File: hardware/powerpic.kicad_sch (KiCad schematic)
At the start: 21 parts

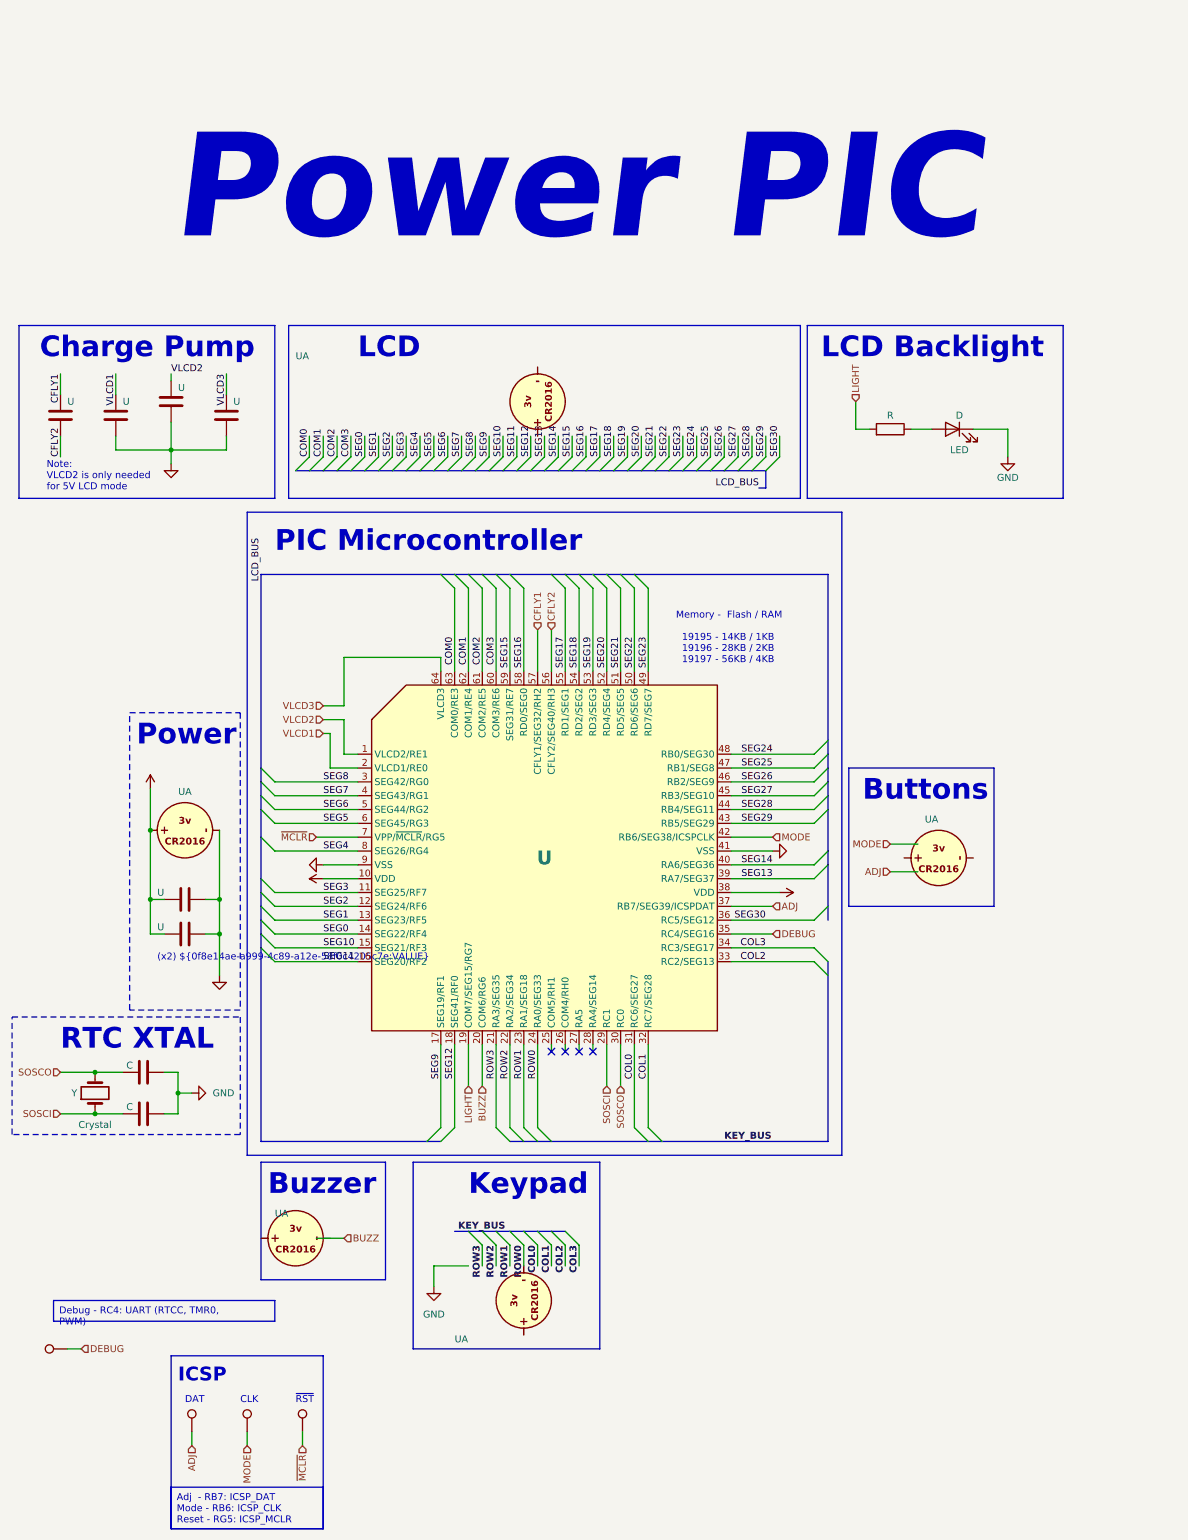
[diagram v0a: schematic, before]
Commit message: release version 2.1
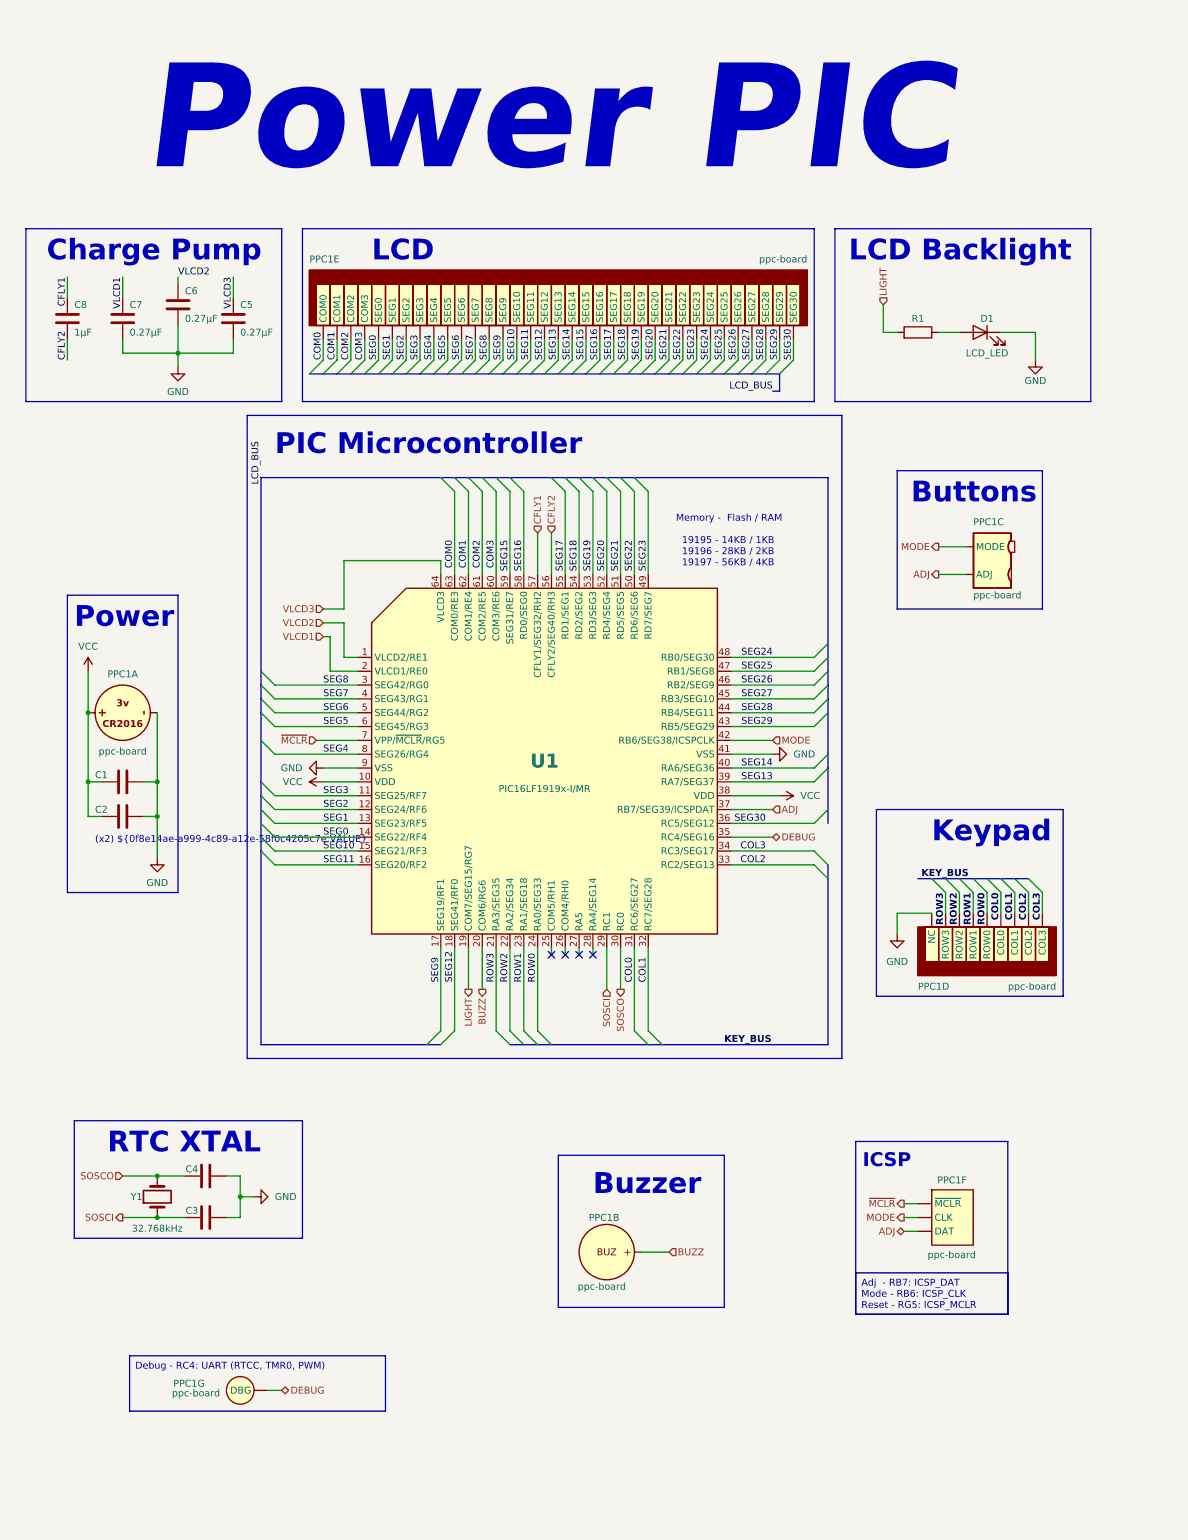
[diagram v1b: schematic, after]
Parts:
- removed TP (x4): TestPoint, symbol Connector:TestPoint
- added unit 7 of PPC1
- added unit 6 of PPC1
- C1, C2: renamed from U; value (none) -> 0.1μF; footprint (none) -> Capacitor_SMD:C_0402_1005Metric
- C3, C4: renamed from C; value C -> TBD; footprint (none) -> Capacitor_SMD:C_0603_1608Metric
- C5, C6, C7: renamed from U; value (none) -> 0.27μF; footprint (none) -> Capacitor_SMD:C_0402_1005Metric
- C8: renamed from U; value (none) -> 1μF; footprint (none) -> Capacitor_SMD:C_0402_1005Metric
- D1: renamed from D; value LED -> LCD_LED; footprint (none) -> LED_SMD:LED_0402_1005Metric
- PPC1: renamed from U; value (none) -> ppc-board; footprint (none) -> ppc-watch:ppc-board
- R1: renamed from R; value R -> TBD; footprint (none) -> Resistor_SMD:R_0603_1608Metric
- U1: renamed from U; value (none) -> PIC16LF1919x-I/MR; footprint (none) -> Package_DFN_QFN:QFN-64-1EP_9x9mm_P0.5mm_EP5.4x5.4mm
- Y1: renamed from Y; value Crystal -> 32.768kHz; footprint (none) -> Crystal:Crystal_SMD_MicroCrystal_CC7V-T1A-2Pin_3.2x1.5mm
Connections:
- net ADJ: now also PPC1.5 (ADJ), PPC1.52 (DAT)
- net BUZZ: now also PPC1.3 (buzz_p)
- net COL0: now also PPC1.11 (COL0)
- net COL1: now also PPC1.12 (COL1)
- net COL2: now also PPC1.13 (COL2)
- net COL3: now also PPC1.14 (COL3)
- net COM0: now also PPC1.15 (COM0)
- net COM1: now also PPC1.16 (COM1)
- net COM2: now also PPC1.17 (COM2)
- net COM3: now also PPC1.18 (COM3)
- net DEBUG: now also PPC1.53 (DBG)
- net GND: now also PPC1.6 (NC)
- net MODE: now also PPC1.4 (MODE), PPC1.51 (CLK)
- net ROW0: now also PPC1.10 (ROW0); no longer PPC1.2 (GND)
- net ROW1: now also PPC1.9 (ROW1)
- net ROW2: now also PPC1.8 (ROW2)
- net ROW3: now also PPC1.7 (ROW3)
- net SEG0: now also PPC1.19 (SEG0)
- net SEG1: now also PPC1.20 (SEG1)
- net SEG10: now also PPC1.29 (SEG10)
- net SEG11: now also PPC1.30 (SEG11)
- net SEG12: now also PPC1.31 (SEG12)
- net SEG13: now also PPC1.32 (SEG13)
- net SEG14: now also PPC1.33 (SEG14)
- net SEG15: now also PPC1.34 (SEG15)
- net SEG16: now also PPC1.35 (SEG16)
- net SEG17: now also PPC1.36 (SEG17)
- net SEG18: now also PPC1.37 (SEG18)
- net SEG19: now also PPC1.38 (SEG19)
- net SEG2: now also PPC1.21 (SEG2)
- net SEG20: now also PPC1.39 (SEG20)
- net SEG21: now also PPC1.40 (SEG21)
- net SEG22: now also PPC1.41 (SEG22)
- net SEG23: now also PPC1.42 (SEG23)
- net SEG24: now also PPC1.43 (SEG24)
- net SEG25: now also PPC1.44 (SEG25)
- net SEG26: now also PPC1.45 (SEG26)
- net SEG27: now also PPC1.46 (SEG27)
- net SEG28: now also PPC1.47 (SEG28)
- net SEG29: now also PPC1.48 (SEG29)
- net SEG3: now also PPC1.22 (SEG3)
- net SEG30: now also PPC1.49 (SEG30)
- net SEG4: now also PPC1.23 (SEG4)
- net SEG5: now also PPC1.24 (SEG5)
- net SEG6: now also PPC1.25 (SEG6)
- net SEG7: now also PPC1.26 (SEG7)
- net SEG8: now also PPC1.27 (SEG8)
- net SEG9: now also PPC1.28 (SEG9)
- net ~{MCLR}: now also PPC1.50 (~{MCLR})
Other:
- note removed: "CLK"
- note removed: "DAT"
- note removed: "Note: VLCD2 is only needed for 5V LCD mode"
- note removed: "~{RST}"
- moved on the sheet: C1, C2, C3, C4, C5, C6, C7, C8, D1, PPC1A, R1, U1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
